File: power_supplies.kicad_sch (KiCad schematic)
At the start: 59 parts, among them Q1 PMOS, Q2 2PNP, U1 ECP5-BGA256, U4 3V3REG, U5 1V15REG, U6 2V5REG, U7 1V8REG

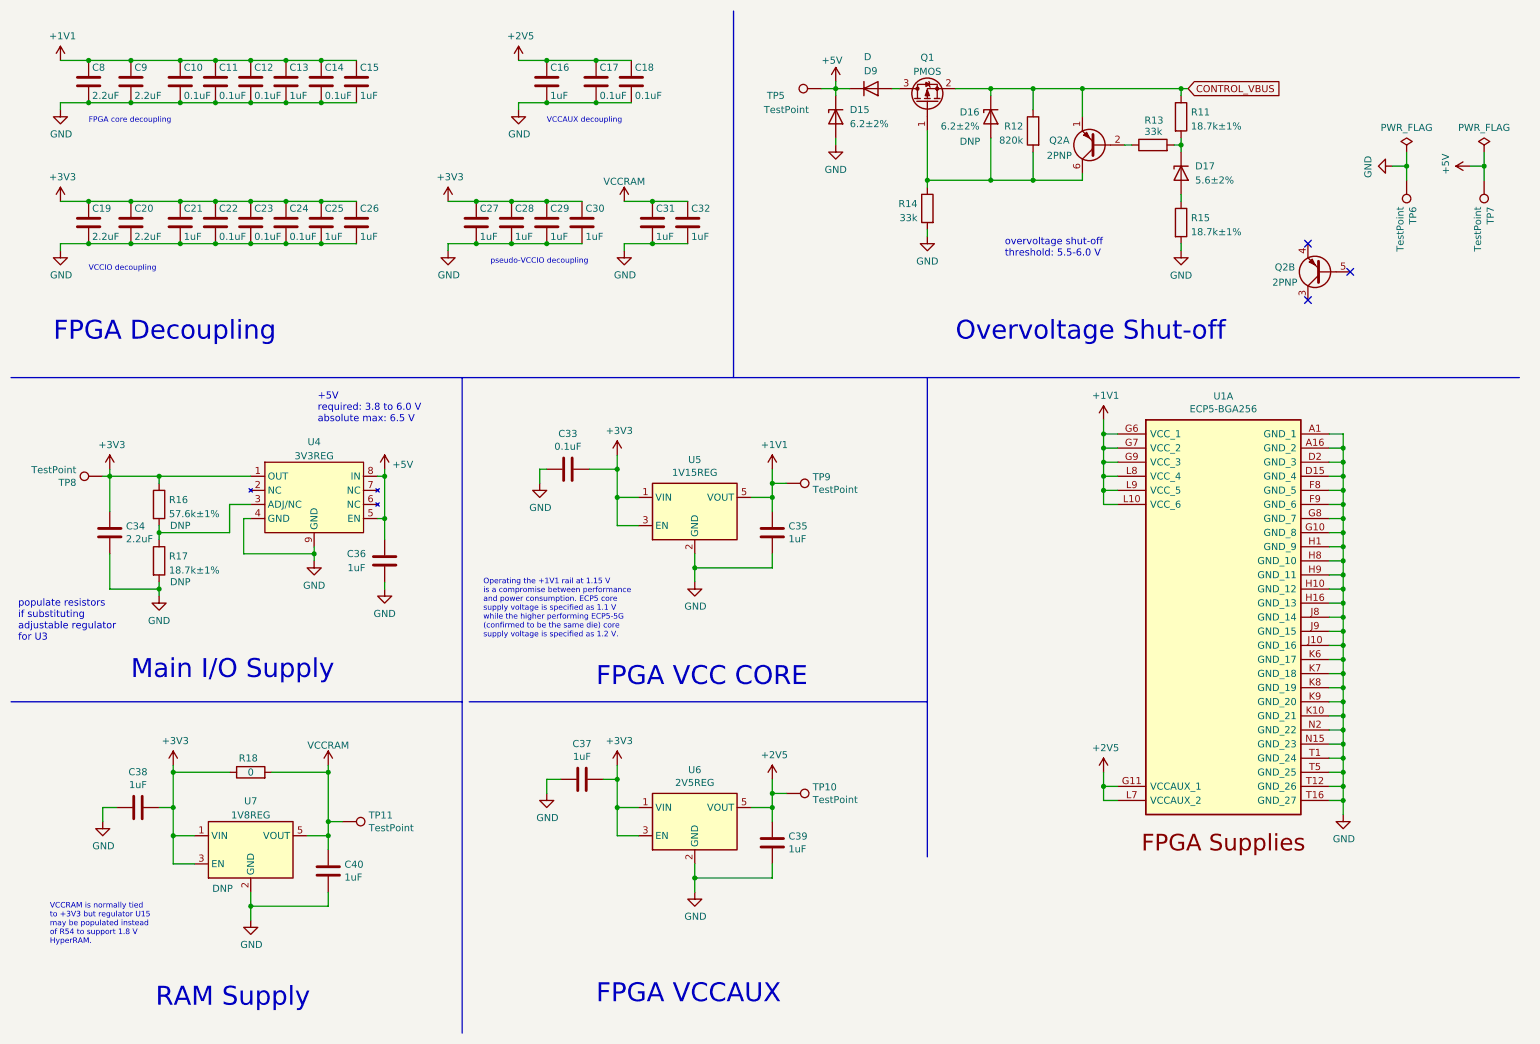
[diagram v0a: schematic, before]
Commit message: schematic wip
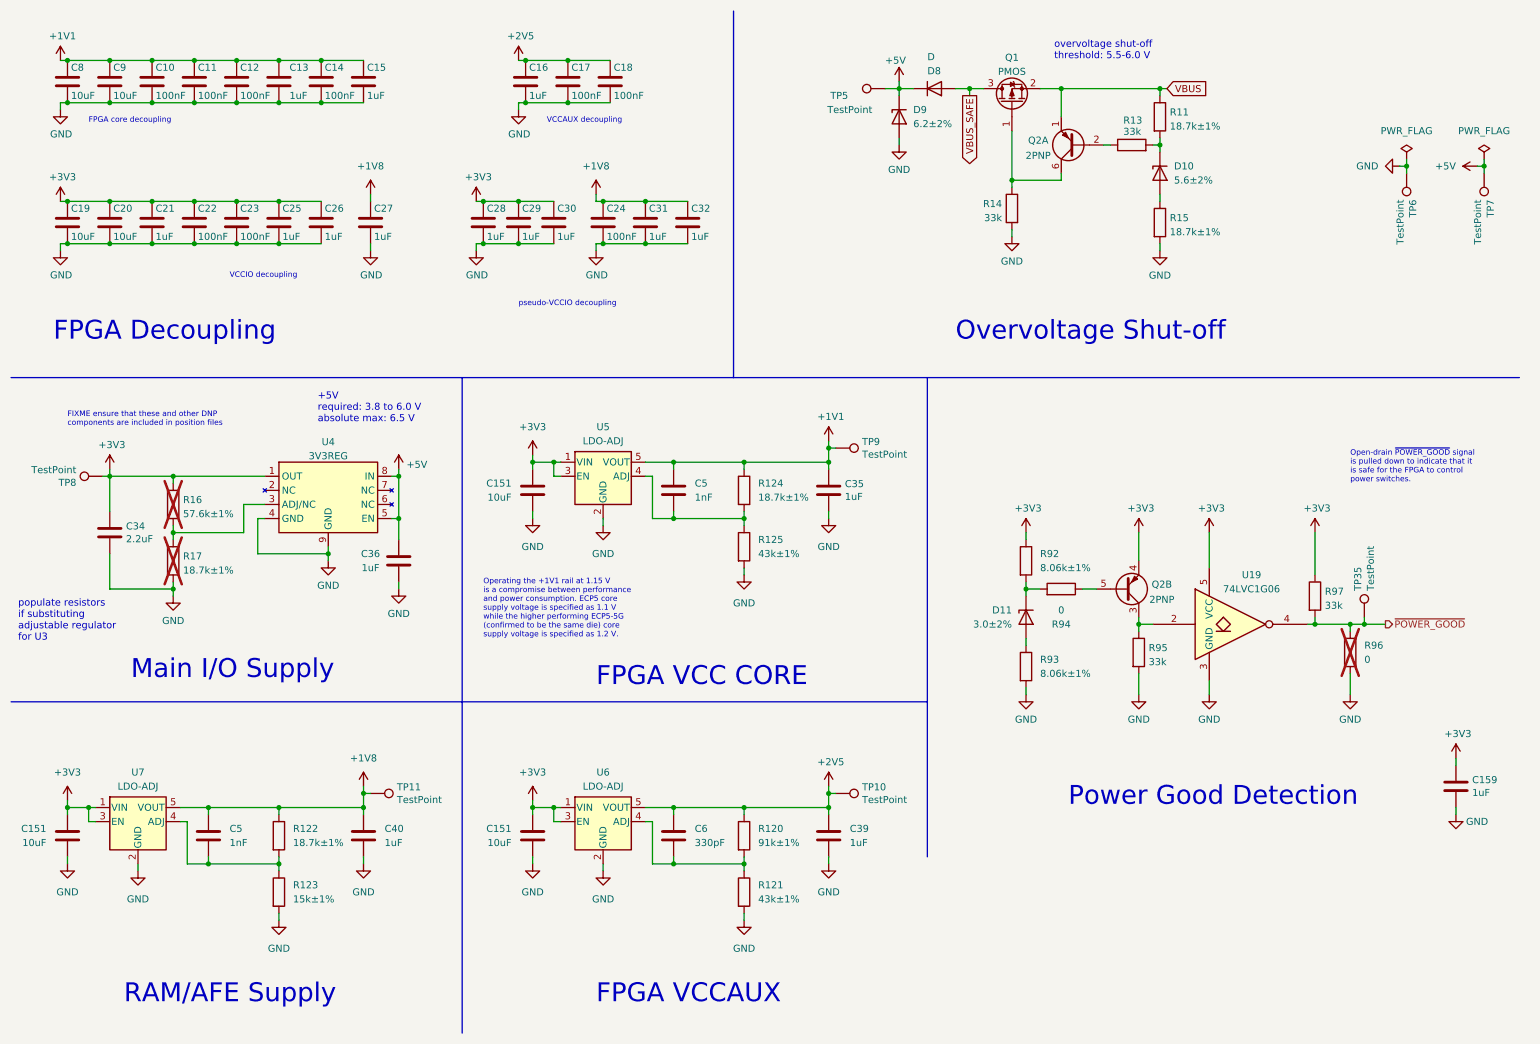
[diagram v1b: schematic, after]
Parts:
- removed C33: 0.1uF, Capacitor_SMD:C_0402_1005Metric, symbol Device:C
- removed C37, C38: 1uF, Capacitor_SMD:C_0402_1005Metric, symbol Device:C
- removed D16: 6.2±2%, mainboard:DFN1006-2, symbol Device:D_Zener
- removed R12: 820k, Resistor_SMD:R_0402_1005Metric, symbol Device:R
- removed R18: 0, Resistor_SMD:R_0402_1005Metric, symbol Device:R
- removed U1: ECP5-BGA256, mainboard:lattice_cabga256, symbol fpgas_and_processors:ECP5-BGA256
- removed U5: 1V15REG, Package_TO_SOT_SMD:SOT-23-5, symbol Regulator_Linear:MIC5504-1.8YM5
- removed U6: 2V5REG, Package_TO_SOT_SMD:SOT-23-5, symbol Regulator_Linear:MIC5504-2.5YM5
- removed U7: 1V8REG, Package_TO_SOT_SMD:SOT-23-5, symbol Regulator_Linear:MIC5504-1.8YM5
- added C151 (x3): 10uF, Capacitor_SMD:C_0603_1608Metric, symbol Device:C
- added C159: 1uF, Capacitor_SMD:C_0402_1005Metric, symbol Device:C
- added C5 (x2): 1nF, Capacitor_SMD:C_0402_1005Metric, symbol Device:C
- added C6: 330pF, Capacitor_SMD:C_0402_1005Metric, symbol Device:C
- added D11: 3.0±2%, cynthion:DFN1006-2, symbol Device:D_Zener
- added R120: 91k±1%, Resistor_SMD:R_0402_1005Metric, symbol Device:R
- added R121, R125: 43k±1%, Resistor_SMD:R_0402_1005Metric, symbol Device:R
- added R122, R124: 18.7k±1%, Resistor_SMD:R_0402_1005Metric, symbol Device:R
- added R123: 15k±1%, Resistor_SMD:R_0402_1005Metric, symbol Device:R
- added R92, R93: 8.06k±1%, Resistor_SMD:R_0402_1005Metric, symbol Device:R
- added R94, R96: 0, Resistor_SMD:R_0402_1005Metric, symbol Device:R
- added R95, R97: 33k, Resistor_SMD:R_0402_1005Metric, symbol Device:R
- added TP35: TestPoint, TestPoint:TestPoint_Pad_D1.0mm, symbol Connector:TestPoint
- added U19: 74LVC1G06, Package_TO_SOT_SMD:SOT-353_SC-70-5, symbol 74xGxx:74LVC1G06
- added U5, U6, U7: LDO-ADJ, Package_TO_SOT_SMD:SOT-23-5, symbol Regulator_Linear:AP2127K-ADJ
- C10, C11, C12, C14, C17, C18, C22, C23, C24: value 0.1uF -> 100nF
- C13, C15, C16, C21, C25, C26, C27, C28, C29, C30, C31, C32, C35, C36, C39, C40: Part Number CL05A105MQ5NNNC -> CL05A105KP5NNNC; Substitution CL05A105KQ5NNNC, CL05A105KP5NNNC, CL05A105KO5NNNC -> any equivalent
- C19, C20, C8, C9: value 2.2uF -> 10uF; Part Number CL10A225KP8NNNC -> CL10A106KP8NNNC
- C34: footprint Capacitor_SMD:C_0603_1608Metric -> Capacitor_SMD:C_0402_1005Metric; Manufacturer Samsung -> Murata; Part Number CL10A225KP8NNNC -> GRM155R61A225KE95D; Substitution any equivalent -> GRM155R61A225*
- R16, R17: DNP DNP -> (none); now not fitted
- renumbered D17 to D10, D9 to D8, D15 to D9
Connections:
- net +1V1: now also C5.1, R124.1, U5.5 (VOUT)
- net +2V5: now also C6.1, R120.1, U6.5 (VOUT)
- net +3V3: now also Q2.4 (E2), C151.1, C151.1, C151.2, C159.1, R92.1, R97.1, U19.5 (VCC), U5.1 (VIN), U5.3 (EN), U6.1 (VIN), U6.3 (EN), U7.1 (VIN), U7.3 (EN); no longer C24.1, C27.1
- net GND: now also C151.1, C151.2, C151.2, C159.2, R121.2, R123.2, R125.2, R93.2, R95.2, R96.1, U19.3 (GND), U5.2 (GND), U6.2 (GND), U7.2 (GND)
- net VBUS_SAFE: now reaches D8.2 (A), Q1.3 (D)
- net at Q2.3 (C2): now also R95.1, U19.2
- net at Q2.5 (B2): now also R94.1
- net CONTROL_VBUS renamed VBUS
- net VCCRAM renamed +1V8
- net +1V8: now also C24.1, C27.1, C5.1, R122.1, U7.5 (VOUT)
- new net: C5.2, R122.2, R123.1, U7.4 (ADJ)
- new net: D11.2 (A), R93.1
- new net: C5.2, R124.2, R125.1, U5.4 (ADJ)
- new net: C6.2, R120.2, R121.1, U6.4 (ADJ)
- new net: D11.1 (K), R92.2, R94.2
- new net ~{POWER_GOOD}: R96.2, R97.2, TP35.1, U19.4
- no-connect marks 3 -> 0
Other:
- note added: "FIXME ensure that these and other DNP components are included in position files"
- note added: "Open-drain ~{POWER_GOOD} signal is pulled down to indicate that it is safe for the FPGA to control power switches."
- note added: "Power Good Detection"
- note added: "RAM/AFE Supply"
- note removed: "RAM Supply"
- note removed: "VCCRAM is normally tied to +3V3 but regulator U15 may be populated instead of R54 to support 1.8 V HyperRAM."
- moved on the sheet: C10, C11, C12, C13, C15, C16, C17, C18, C19, C20, C21, C22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
